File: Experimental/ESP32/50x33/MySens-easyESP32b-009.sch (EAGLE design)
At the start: 22 parts, among them U2 RFM69HCW, U3 ESP-WROOM-32

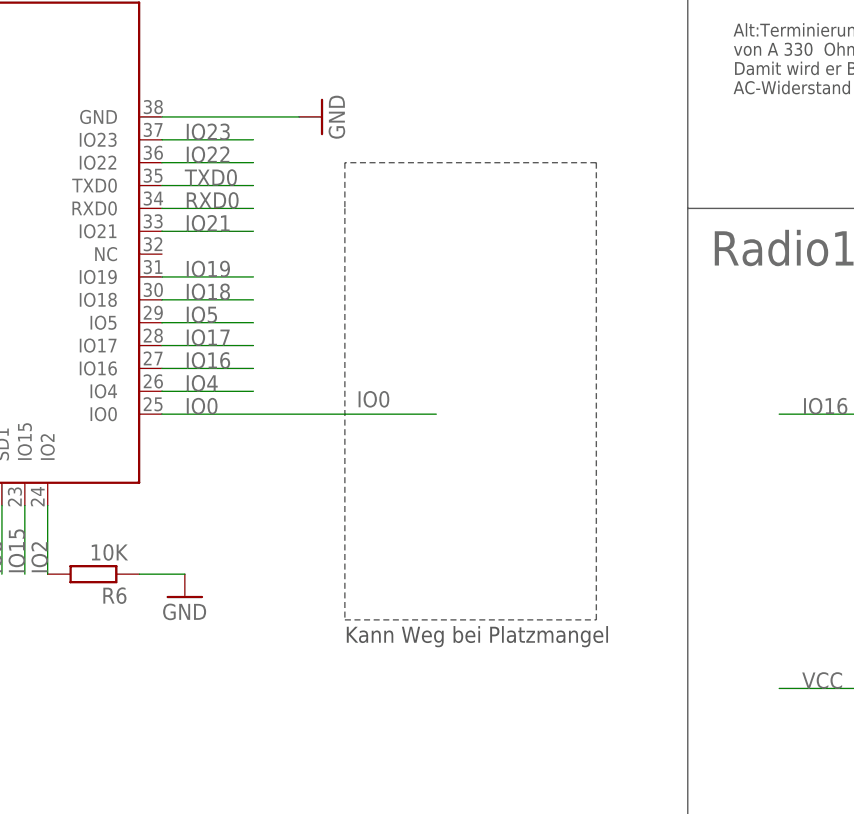
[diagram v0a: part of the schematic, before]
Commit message: ESP32 AddOn
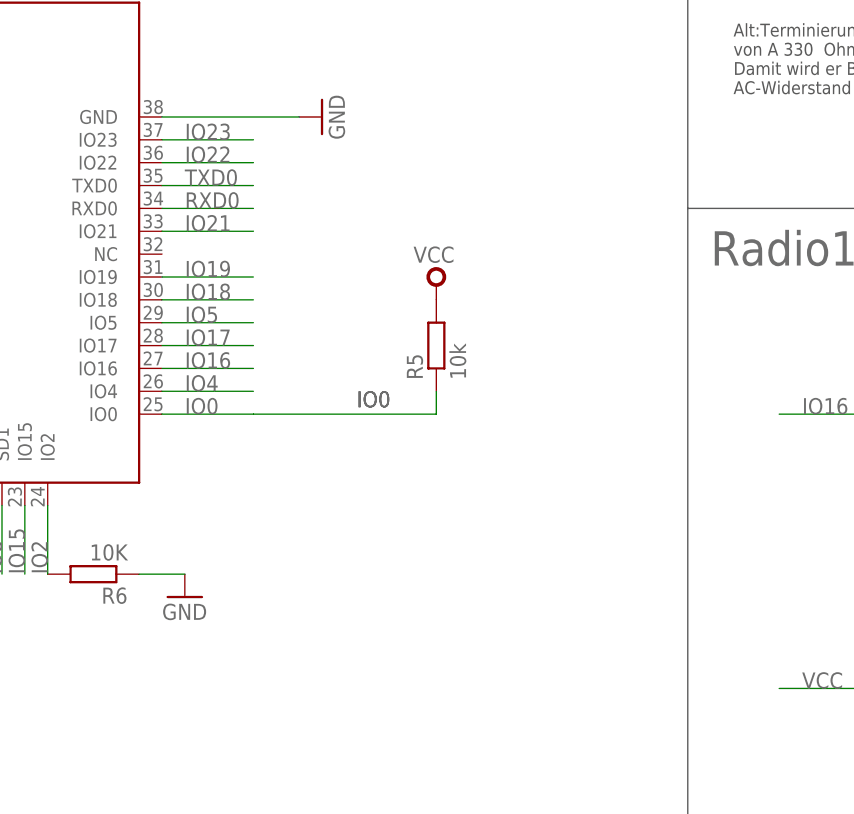
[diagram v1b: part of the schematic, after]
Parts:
- added R5: 10k, rcl:R-EU_R0603
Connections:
- net IO0: now also R5.1
- net VCC: now also R5.2
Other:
- note removed: "Kann Weg bei Platzmangel"
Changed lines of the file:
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@@
 <?xml version="1.0" encoding="utf-8"?>
 <!DOCTYPE eagle SYSTEM "eagle.dtd">
-<eagle version="7.7.0">
+<eagle version="7.6.0">
 <drawing>
 <settings>
@@
 <part name="ANT2" library="pinhead" deviceset="PINHD-1X1" device=""/>
 <part name="R7" library="rcl" deviceset="R-EU_" device="M0805" value="100k"/>
+<part name="V1" library="supply" deviceset="VCC" device=""/>
+<part name="R5" library="rcl" deviceset="R-EU_" device="R0603" value="10k"/>
 </parts>
 <sheets>
@@
 <circle x="152.4" y="27.94" radius="2.54" width="0.1524" layer="102"/>
 <text x="137.16" y="55.88" size="5.08" layer="102">???? io5 ???</text>
-<wire x1="15.24" y1="73.66" x2="15.24" y2="27.94" width="0.1524" layer="97" style="shortdash"/>
-<wire x1="15.24" y1="27.94" x2="43.18" y2="27.94" width="0.1524" layer="97" style="shortdash"/>
-<wire x1="43.18" y1="27.94" x2="43.18" y2="78.74" width="0.1524" layer="97" style="shortdash"/>
-<wire x1="43.18" y1="78.74" x2="15.24" y2="78.74" width="0.1524" layer="97" style="shortdash"/>
-<wire x1="15.24" y1="78.74" x2="15.24" y2="73.66" width="0.1524" layer="97" style="shortdash"/>
-<text x="15.24" y="25.4" size="1.778" layer="97">Kann Weg bei Platzmangel</text>
 <text x="-63.5" y="-55.88" size="1.778" layer="97">Wenn man die Pins von dem MYSx Stecker: 3.3V, GND, RX, TX, EN und GPIO00
 nimmt und einen Standad USB Programmer (z.B. einen FDDI um 1,60€) nimmt und den
@@
 <instance part="ANT2" gate="G$1" x="223.52" y="30.48"/>
 <instance part="R7" gate="G$1" x="-55.88" y="-142.24" rot="R180"/>
+<instance part="V1" gate="VCC" x="25.4" y="66.04"/>
+<instance part="R5" gate="G$1" x="25.4" y="58.42" rot="R90"/>
 </instances>
 <busses>
@@
 <label x="-81.28" y="-119.38" size="1.778" layer="95"/>
 </segment>
+<segment>
+<pinref part="V1" gate="VCC" pin="VCC"/>
+<pinref part="R5" gate="G$1" pin="2"/>
+</segment>
 </net>
 <net name="A4" class="0">
@@
 <label x="-2.54" y="50.8" size="1.778" layer="95"/>
 <pinref part="U3" gate="G$1" pin="IO0"/>
-<wire x1="-5.08" y1="50.8" x2="25.4" y2="50.8" width="0.1524" layer="91"/>
+<wire x1="-5.08" y1="50.8" x2="5.08" y2="50.8" width="0.1524" layer="91"/>
 <label x="20.32" y="53.34" size="1.778" layer="95" rot="R180"/>
-</segment>
-<segment>
+<pinref part="R5" gate="G$1" pin="1"/>
+<label x="20.32" y="53.34" size="1.778" layer="95" rot="R180"/>
+<wire x1="25.4" y1="50.8" x2="25.4" y2="53.34" width="0.1524" layer="91"/>
+<wire x1="5.08" y1="50.8" x2="25.4" y2="50.8" width="0.1524" layer="91"/>
+</segment>
+<segment>
